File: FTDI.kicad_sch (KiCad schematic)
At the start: 30 parts, among them J301 Conn_02x06_Odd_Even, J302 Conn_01x04_Male, U301 FT2232HL, U302 93LC56BT-I/OT, Y301 12MHz

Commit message: Update 7/30
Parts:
- J302: footprint Connector_PinHeader_2.54mm:PinHeader_1x04_P2.54mm_Horizontal -> Connector_PinHeader_2.54mm:PinHeader_1x04_P2.54mm_Vertical
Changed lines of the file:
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@@
     (property "Reference" "J302" (id 0) (at 271.78 31.115 0))
     (property "Value" "Conn_01x04_Male" (id 1) (at 271.78 33.655 0))
-    (property "Footprint" "Connector_PinHeader_2.54mm:PinHeader_1x04_P2.54mm_Horizontal" (id 2) (at 271.145 39.37 0)
+    (property "Footprint" "Connector_PinHeader_2.54mm:PinHeader_1x04_P2.54mm_Vertical" (id 2) (at 271.145 39.37 0)
       (effects (font (size 1.27 1.27)) hide)
     )

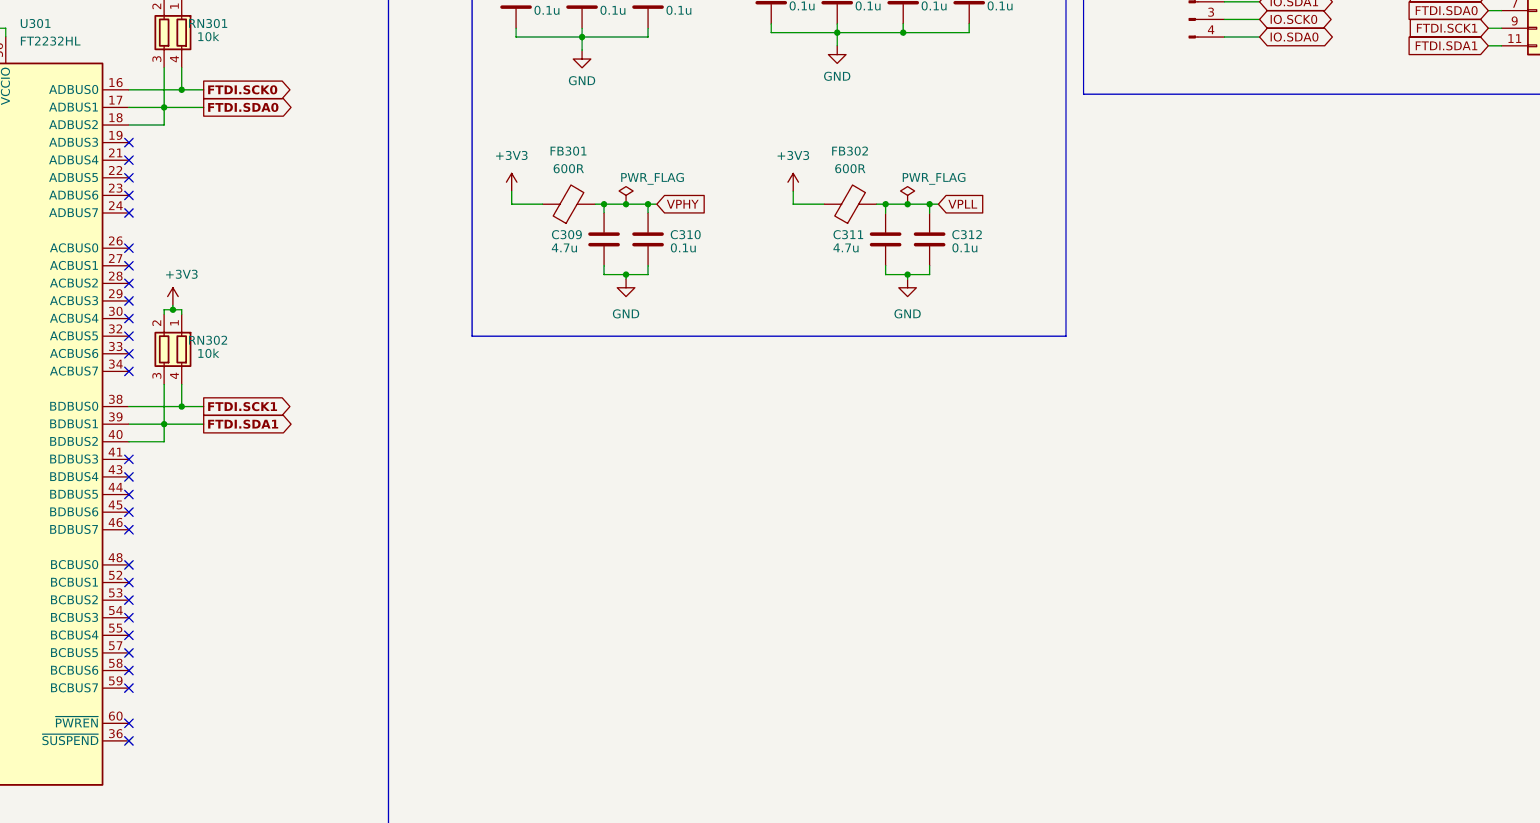
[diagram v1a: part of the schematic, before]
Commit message: Update 8/2
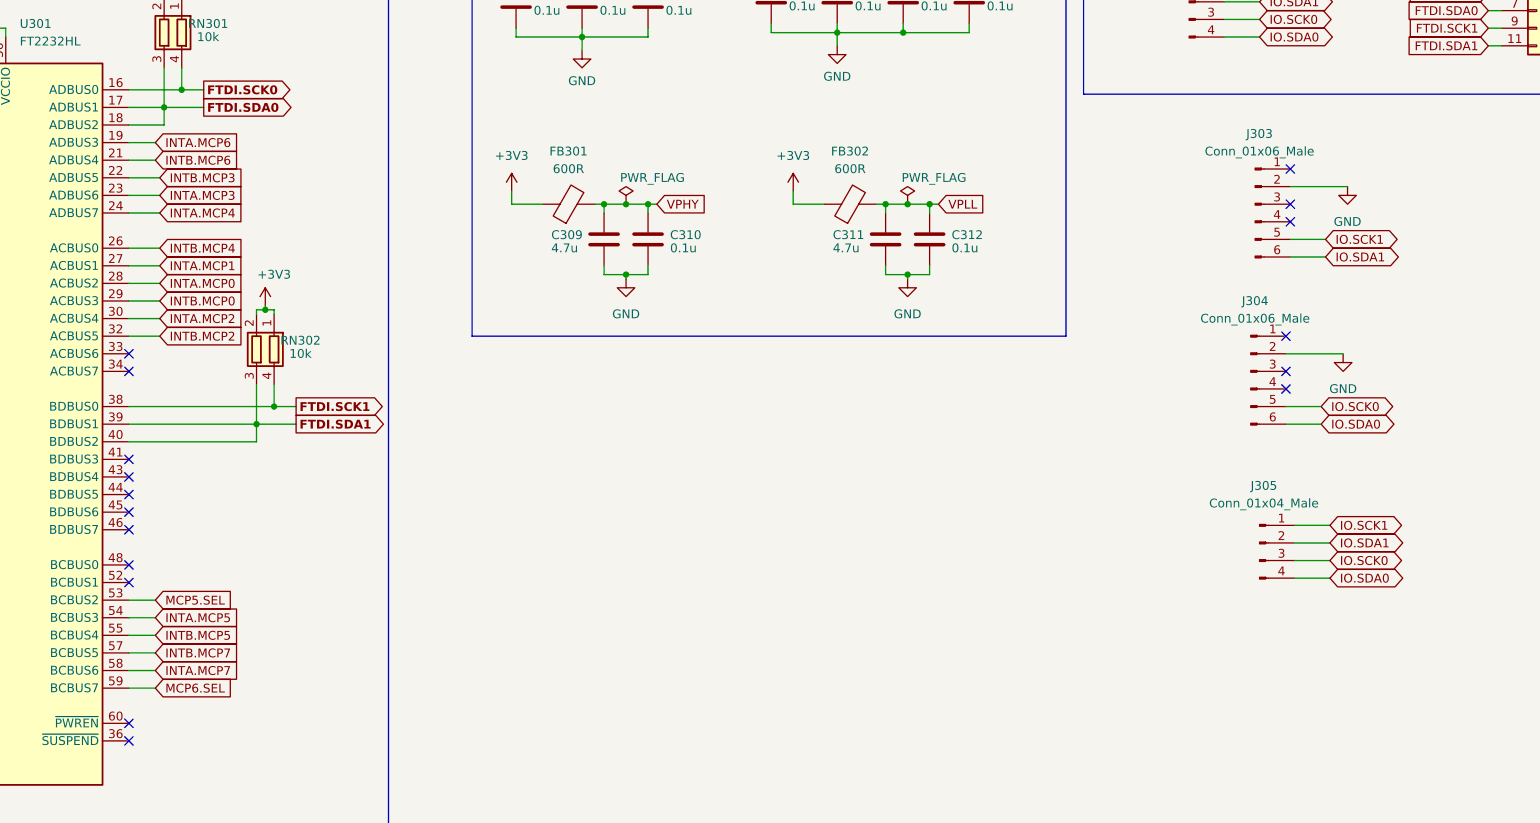
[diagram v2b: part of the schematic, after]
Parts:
- added J303, J304: Conn_01x06_Male, Connector_PinHeader_2.54mm:PinHeader_1x06_P2.54mm_Vertical, symbol Connector:Conn_01x06_Male
- added J305: Conn_01x04_Male, Connector_PinHeader_2.54mm:PinHeader_1x04_P2.54mm_Horizontal, symbol Connector:Conn_01x04_Male
- J302: footprint Connector_PinHeader_2.54mm:PinHeader_1x04_P2.54mm_Vertical -> Connector_PinHeader_2.54mm:PinHeader_1x04_P2.54mm_Horizontal
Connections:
- net GND: now also J303.2 (Pin_2), J304.2 (Pin_2)
- net IO.SCK0: now also J304.5 (Pin_5), J305.3 (Pin_3)
- net IO.SCK1: now also J303.5 (Pin_5), J305.1 (Pin_1)
- net IO.SDA0: now also J304.6 (Pin_6), J305.4 (Pin_4)
- net IO.SDA1: now also J303.6 (Pin_6), J305.2 (Pin_2)
- net INTA.MCP6: now reaches U301.19 (ADBUS3)
- net INTB.MCP6: now reaches U301.21 (ADBUS4)
- net INTB.MCP3: now reaches U301.22 (ADBUS5)
- net INTA.MCP3: now reaches U301.23 (ADBUS6)
- net INTA.MCP4: now reaches U301.24 (ADBUS7)
- net INTB.MCP4: now reaches U301.26 (ACBUS0)
- net INTA.MCP1: now reaches U301.27 (ACBUS1)
- net INTA.MCP0: now reaches U301.28 (ACBUS2)
- net INTB.MCP0: now reaches U301.29 (ACBUS3)
- net INTA.MCP2: now reaches U301.30 (ACBUS4)
- net INTB.MCP2: now reaches U301.32 (ACBUS5)
- net MCP5.SEL: now reaches U301.53 (BCBUS2)
- net INTA.MCP5: now reaches U301.54 (BCBUS3)
- net INTB.MCP5: now reaches U301.55 (BCBUS4)
- net INTB.MCP7: now reaches U301.57 (BCBUS5)
- net INTA.MCP7: now reaches U301.58 (BCBUS6)
- net MCP6.SEL: now reaches U301.59 (BCBUS7)
- no-connect marks 28 -> 17
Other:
- moved on the sheet: RN302

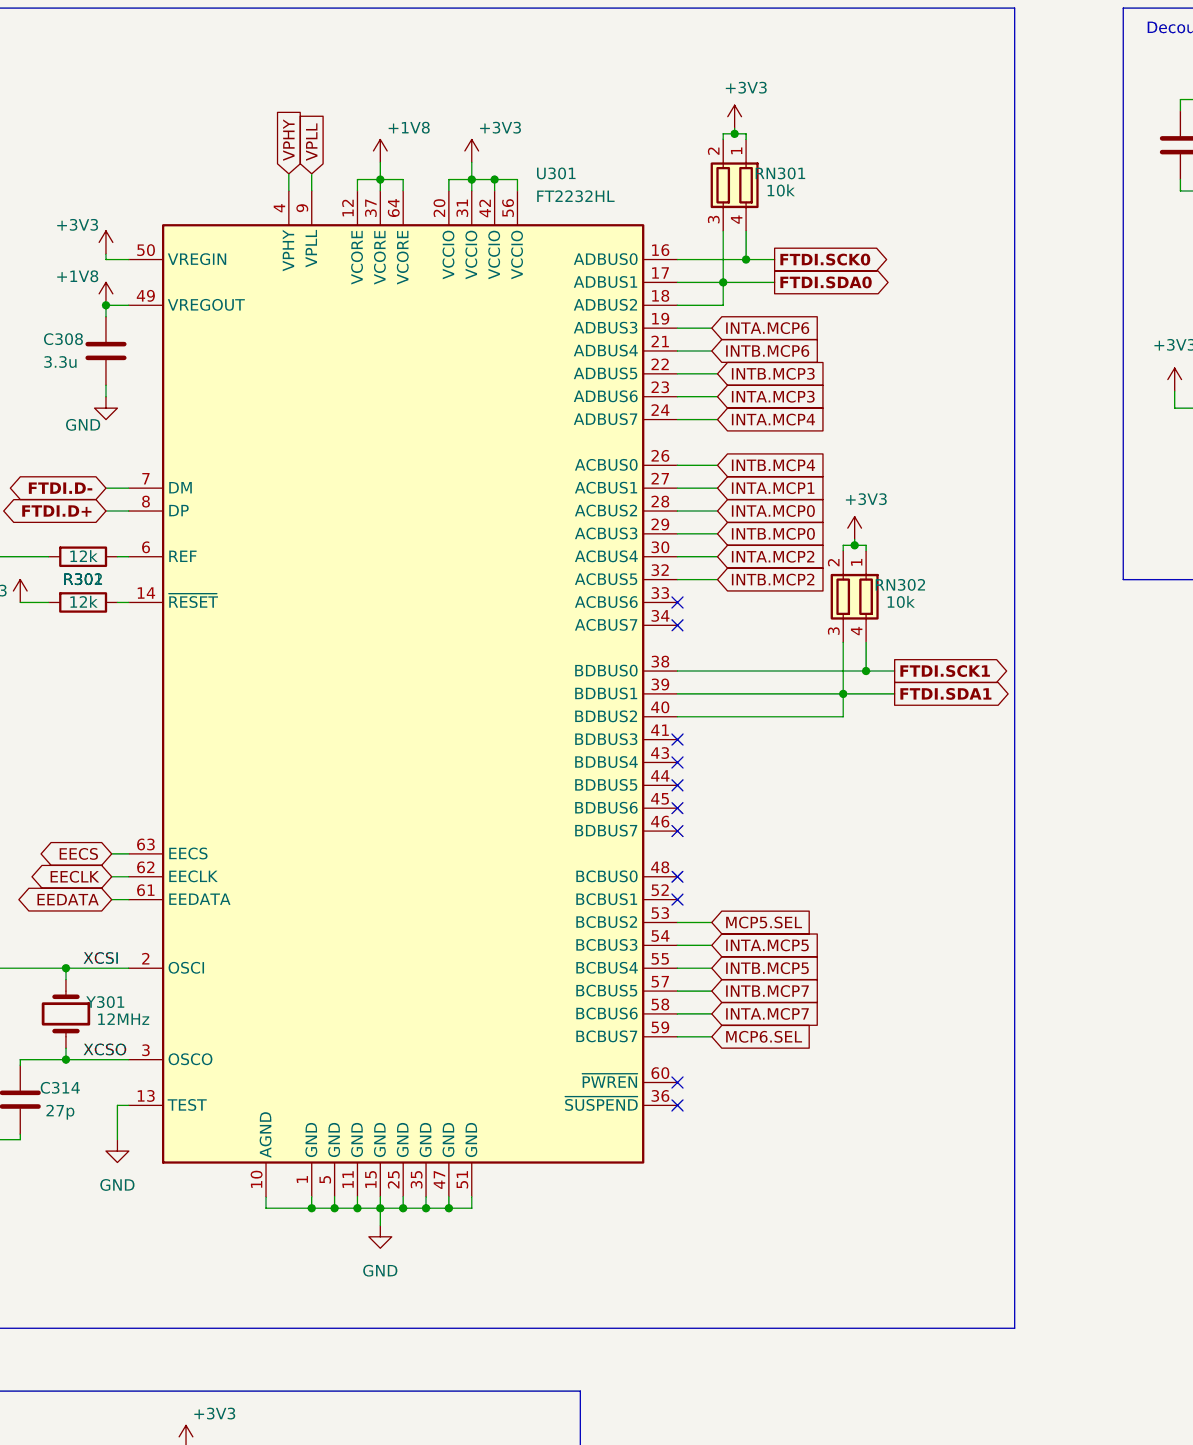
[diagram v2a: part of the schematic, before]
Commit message: Complete Design v2
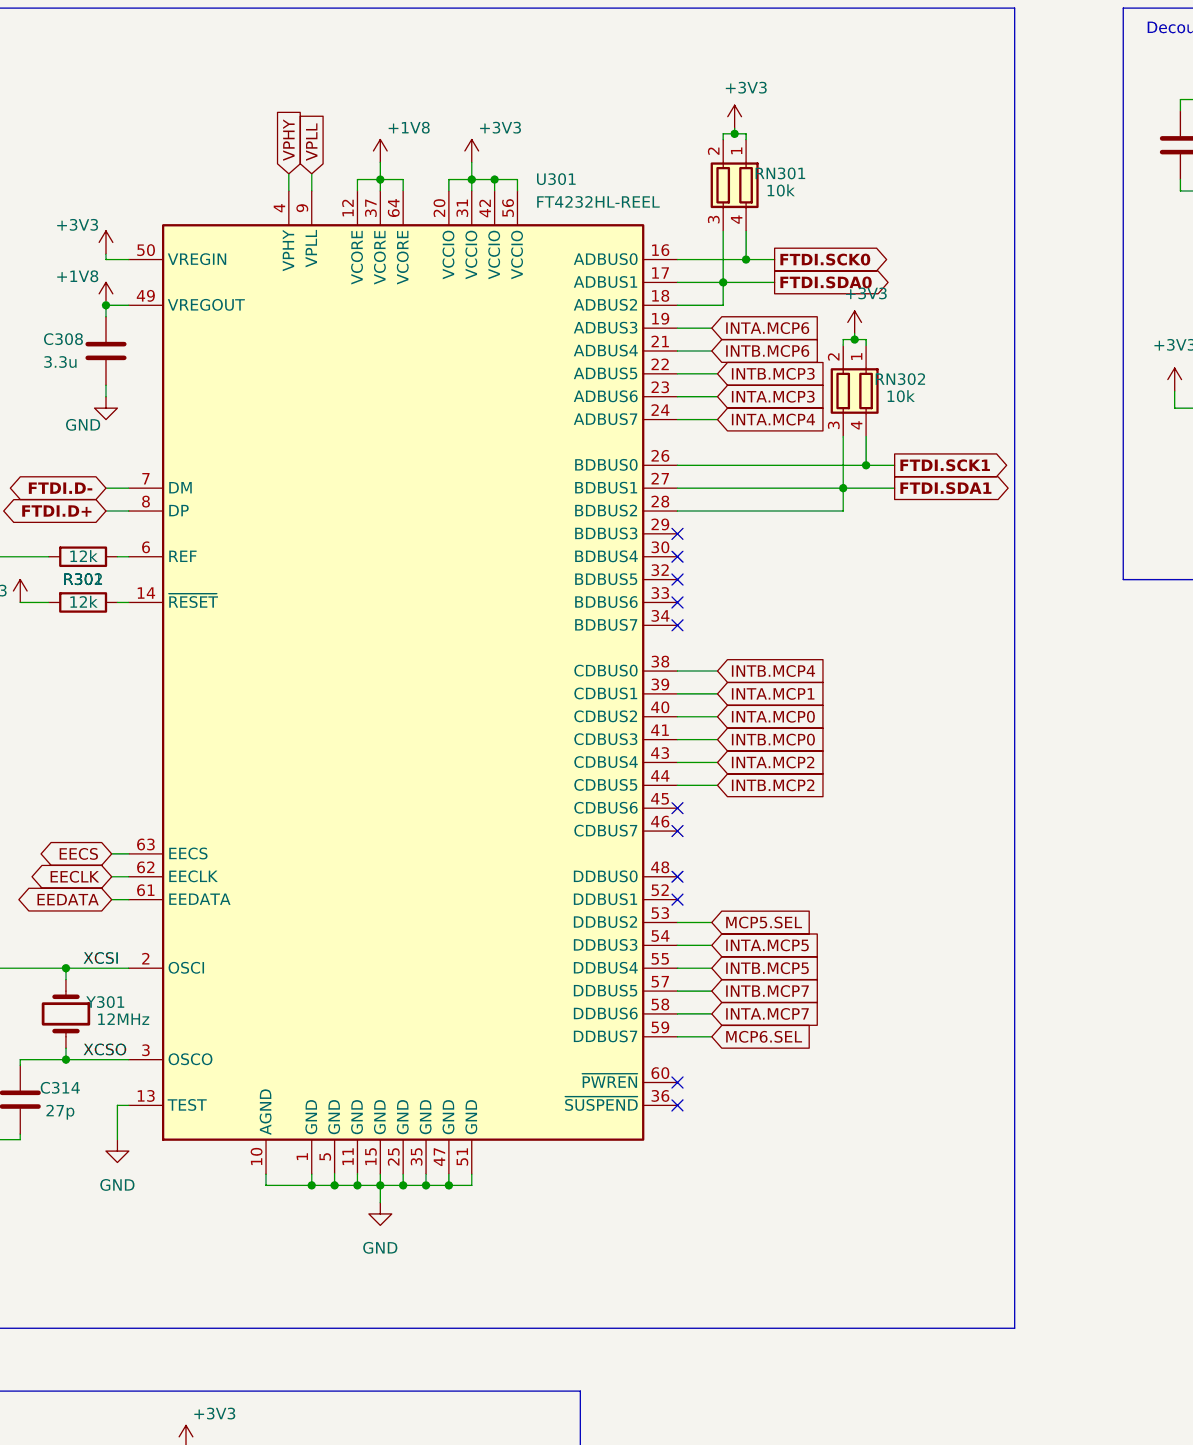
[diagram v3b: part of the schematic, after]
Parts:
- J301: LCSC (none) -> C5224012; LCSC Part Number (none) -> C5224012
- J302, J305: LCSC (none) -> C91552; LCSC Part Number (none) -> C91552
- J303, J304: footprint Connector_PinHeader_2.54mm:PinHeader_1x06_P2.54mm_Vertical -> Connector_PinSocket_2.54mm:PinSocket_1x06_P2.54mm_Vertical; LCSC (none) -> C5224026; LCSC Part Number (none) -> C5224026
- U301: value FT2232HL -> FT4232HL-REEL; symbol Interface_USB:FT2232HL -> Interface_USB:FT4232H; LCSC C27882 -> C56742; LCSC Part Number C27882 -> C56742
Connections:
- net FTDI.SCK1: now also U301.26 (BDBUS0); no longer U301.38 (BDBUS0)
- net FTDI.SDA1: now also U301.27 (BDBUS1), U301.28 (BDBUS2); no longer U301.39 (BDBUS1), U301.40 (BDBUS2)
- net INTA.MCP0: now also U301.40 (CDBUS2); no longer U301.28 (ACBUS2)
- net INTA.MCP1: now also U301.39 (CDBUS1); no longer U301.27 (ACBUS1)
- net INTA.MCP2: now also U301.43 (CDBUS4); no longer U301.30 (ACBUS4)
- net INTB.MCP0: now also U301.41 (CDBUS3); no longer U301.29 (ACBUS3)
- net INTB.MCP2: now also U301.44 (CDBUS5); no longer U301.32 (ACBUS5)
- net INTB.MCP4: now also U301.38 (CDBUS0); no longer U301.26 (ACBUS0)
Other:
- moved on the sheet: U301
